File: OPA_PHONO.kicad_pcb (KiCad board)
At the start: 4 copper layers, 100 x 15 mm, 62 parts, among them J1 PJRAS2X1S01X, J2 PJRAS2X1S01X, J3 UJC-HP-3-SMT-TR, U1 OPA1644AxD, U2 OPA1612AxD, U3 LTC3265xDHC

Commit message: change output resistor to 499R
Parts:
- R12, R15, R24, R3, R6, R8: value 68R -> 499R
- R14, R19, R2, R7: value 2.32k -> 16k
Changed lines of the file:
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@@
     (descr "Resistor SMD 0402 (1005 Metric), square (rectangular) end terminal, IPC_7351 nominal, (Body size source: IPC-SM-782 page 72, https://www.pcb-3d.com/wordpress/wp-content/uploads/ipc-sm-782a_amendment_1_and_2.pdf), generated with kicad-footprint-generator")
     (tags "resistor")
-    (property "Description" "RES SMD 68 OHM 1% 1/16W 0402")
-    (property "MPN" "RT0402FRE0768RL")
+    (property "Description" "RES SMD 499R OHM 1% 1/16W 0402")
+    (property "MPN" "RT0402FRE07499RL")
     (property "Manufacturer" "YAGEO")
     (property "Sheetfile" "RIAA_PHONO.kicad_sch")
@@
       (effects (font (size 1 1) (thickness 0.15)))
     )
-    (fp_text value "68R" (at 0 1.17) (layer "F.Fab")
+    (fp_text value "499R" (at 0 1.17) (layer "F.Fab")
       (effects (font (size 1 1) (thickness 0.15)))
     )
@@
     (descr "Resistor SMD 0402 (1005 Metric), square (rectangular) end terminal, IPC_7351 nominal, (Body size source: IPC-SM-782 page 72, https://www.pcb-3d.com/wordpress/wp-content/uploads/ipc-sm-782a_amendment_1_and_2.pdf), generated with kicad-footprint-generator")
     (tags "resistor")
-    (property "Description" "RES SMD 2.32K OHM 1% 1/16W 0402")
-    (property "MPN" "RT0402FRE072K32L")
+    (property "Description" "RES SMD 16K OHM 1% 1/16W 0402")
+    (property "MPN" "RT0402FRE0716KL")
     (property "Manufacturer" "YAGEO")
     (property "Sheetfile" "RIAA_PHONO.kicad_sch")
@@
       (effects (font (size 1 1) (thickness 0.15)))
     )
-    (fp_text value "2.32k" (at 0 1.17 90) (layer "F.Fab")
+    (fp_text value "16k" (at 0 1.17 90) (layer "F.Fab")
       (effects (font (size 1 1) (thickness 0.15)))
     )
@@
     (descr "Resistor SMD 0402 (1005 Metric), square (rectangular) end terminal, IPC_7351 nominal, (Body size source: IPC-SM-782 page 72, https://www.pcb-3d.com/wordpress/wp-content/uploads/ipc-sm-782a_amendment_1_and_2.pdf), generated with kicad-footprint-generator")
     (tags "resistor")
-    (property "Description" "RES SMD 68 OHM 1% 1/16W 0402")
-    (property "MPN" "RT0402FRE0768RL")
+    (property "Description" "RES SMD 499R OHM 1% 1/16W 0402")
+    (property "MPN" "RT0402FRE07499RL")
     (property "Manufacturer" "YAGEO")
     (property "Sheetfile" "RIAA_PHONO.kicad_sch")
@@
       (effects (font (size 1 1) (thickness 0.15)))
     )
-    (fp_text value "68R" (at 0 1.17) (layer "F.Fab")
+    (fp_text value "499R" (at 0 1.17) (layer "F.Fab")
       (effects (font (size 1 1) (thickness 0.15)))
     )
@@
     (descr "Resistor SMD 0402 (1005 Metric), square (rectangular) end terminal, IPC_7351 nominal, (Body size source: IPC-SM-782 page 72, https://www.pcb-3d.com/wordpress/wp-content/uploads/ipc-sm-782a_amendment_1_and_2.pdf), generated with kicad-footprint-generator")
     (tags "resistor")
-    (property "Description" "RES SMD 2.32K OHM 1% 1/16W 0402")
-    (property "MPN" "RT0402FRE072K32L")
+    (property "Description" "RES SMD 16K OHM 1% 1/16W 0402")
+    (property "MPN" "RT0402FRE0716KL")
     (property "Manufacturer" "YAGEO")
     (property "Sheetfile" "RIAA_PHONO.kicad_sch")
@@
       (effects (font (size 1 1) (thickness 0.15)))
     )
-    (fp_text value "2.32k" (at 0 1.17) (layer "F.Fab")
+    (fp_text value "16k" (at 0 1.17) (layer "F.Fab")
       (effects (font (size 1 1) (thickness 0.15)))
     )
@@
     (descr "Resistor SMD 0402 (1005 Metric), square (rectangular) end terminal, IPC_7351 nominal, (Body size source: IPC-SM-782 page 72, https://www.pcb-3d.com/wordpress/wp-content/uploads/ipc-sm-782a_amendment_1_and_2.pdf), generated with kicad-footprint-generator")
     (tags "resistor")
-    (property "Description" "RES SMD 68 OHM 1% 1/16W 0402")
-    (property "MPN" "RT0402FRE0768RL")
+    (property "Description" "RES SMD 499R OHM 1% 1/16W 0402")
+    (property "MPN" "RT0402FRE07499RL")
     (property "Manufacturer" "YAGEO")
     (property "Sheetfile" "RIAA_PHONO.kicad_sch")
@@
       (effects (font (size 1 1) (thickness 0.15)))
     )
-    (fp_text value "68R" (at 0 1.17) (layer "F.Fab")
+    (fp_text value "499R" (at 0 1.17) (layer "F.Fab")
       (effects (font (size 1 1) (thickness 0.15)))
     )
@@
     (descr "Resistor SMD 0402 (1005 Metric), square (rectangular) end terminal, IPC_7351 nominal, (Body size source: IPC-SM-782 page 72, https://www.pcb-3d.com/wordpress/wp-content/uploads/ipc-sm-782a_amendment_1_and_2.pdf), generated with kicad-footprint-generator")
     (tags "resistor")
-    (property "Description" "RES SMD 68 OHM 1% 1/16W 0402")
-    (property "MPN" "RT0402FRE0768RL")
+    (property "Description" "RES SMD 499R OHM 1% 1/16W 0402")
+    (property "MPN" "RT0402FRE07499RL")
     (property "Manufacturer" "YAGEO")
     (property "Sheetfile" "RIAA_PHONO.kicad_sch")
@@
       (effects (font (size 1 1) (thickness 0.15)))
     )
-    (fp_text value "68R" (at 0 1.17 90) (layer "F.Fab")
+    (fp_text value "499R" (at 0 1.17 90) (layer "F.Fab")
       (effects (font (size 1 1) (thickness 0.15)))
     )
@@
     (descr "Resistor SMD 0402 (1005 Metric), square (rectangular) end terminal, IPC_7351 nominal, (Body size source: IPC-SM-782 page 72, https://www.pcb-3d.com/wordpress/wp-content/uploads/ipc-sm-782a_amendment_1_and_2.pdf), generated with kicad-footprint-generator")
     (tags "resistor")
-    (property "Description" "RES SMD 2.32K OHM 1% 1/16W 0402")
-    (property "MPN" "RT0402FRE072K32L")
+    (property "Description" "RES SMD 16K OHM 1% 1/16W 0402")
+    (property "MPN" "RT0402FRE0716KL")
     (property "Manufacturer" "YAGEO")
     (property "Sheetfile" "RIAA_PHONO.kicad_sch")
@@
       (effects (font (size 1 1) (thickness 0.15)))
     )
-    (fp_text value "2.32k" (at 0 1.17) (layer "F.Fab")
+    (fp_text value "16k" (at 0 1.17) (layer "F.Fab")
       (effects (font (size 1 1) (thickness 0.15)))
     )
@@
     (descr "Resistor SMD 0402 (1005 Metric), square (rectangular) end terminal, IPC_7351 nominal, (Body size source: IPC-SM-782 page 72, https://www.pcb-3d.com/wordpress/wp-content/uploads/ipc-sm-782a_amendment_1_and_2.pdf), generated with kicad-footprint-generator")
     (tags "resistor")
-    (property "Description" "RES SMD 68 OHM 1% 1/16W 0402")
-    (property "MPN" "RT0402FRE0768RL")
+    (property "Description" "RES SMD 499R OHM 1% 1/16W 0402")
+    (property "MPN" "RT0402FRE07499RL")
     (property "Manufacturer" "YAGEO")
     (property "Sheetfile" "RIAA_PHONO.kicad_sch")
@@
       (effects (font (size 1 1) (thickness 0.15)))
     )
-    (fp_text value "68R" (at 0 1.17) (layer "F.Fab")
+    (fp_text value "499R" (at 0 1.17) (layer "F.Fab")
       (effects (font (size 1 1) (thickness 0.15)))
     )
@@
     (descr "Resistor SMD 0402 (1005 Metric), square (rectangular) end terminal, IPC_7351 nominal, (Body size source: IPC-SM-782 page 72, https://www.pcb-3d.com/wordpress/wp-content/uploads/ipc-sm-782a_amendment_1_and_2.pdf), generated with kicad-footprint-generator")
     (tags "resistor")
-    (property "Description" "RES SMD 68 OHM 1% 1/16W 0402")
-    (property "MPN" "RT0402FRE0768RL")
+    (property "Description" "RES SMD 499R OHM 1% 1/16W 0402")
+    (property "MPN" "RT0402FRE07499RL")
     (property "Manufacturer" "YAGEO")
     (property "Sheetfile" "RIAA_PHONO.kicad_sch")
@@
       (effects (font (size 1 1) (thickness 0.15)))
     )
-    (fp_text value "68R" (at 0 1.17 90) (layer "F.Fab")
+    (fp_text value "499R" (at 0 1.17 90) (layer "F.Fab")
       (effects (font (size 1 1) (thickness 0.15)))
     )
@@
     (descr "Resistor SMD 0402 (1005 Metric), square (rectangular) end terminal, IPC_7351 nominal, (Body size source: IPC-SM-782 page 72, https://www.pcb-3d.com/wordpress/wp-content/uploads/ipc-sm-782a_amendment_1_and_2.pdf), generated with kicad-footprint-generator")
     (tags "resistor")
-    (property "Description" "RES SMD 2.32K OHM 1% 1/16W 0402")
-    (property "MPN" "RT0402FRE072K32L")
+    (property "Description" "RES SMD 16K OHM 1% 1/16W 0402")
+    (property "MPN" "RT0402FRE0716KL")
     (property "Manufacturer" "YAGEO")
     (property "Sheetfile" "RIAA_PHONO.kicad_sch")
@@
       (effects (font (size 1 1) (thickness 0.15)))
     )
-    (fp_text value "2.32k" (at 0 1.17 90) (layer "F.Fab")
-      (effects (font (size 1 1) (thickness 0.15)))
-    )
+    (fp_text value "16k" (at 0 1.17 90) (layer "F.Fab")
+      (effects (font (size 1 1) (thickness 0.15)))
+    )

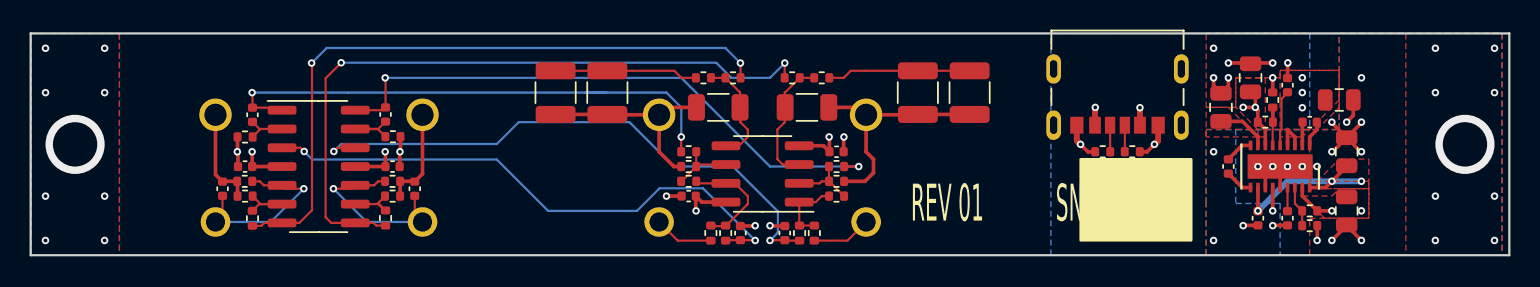
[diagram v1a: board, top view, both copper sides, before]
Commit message: Generate Gerbers
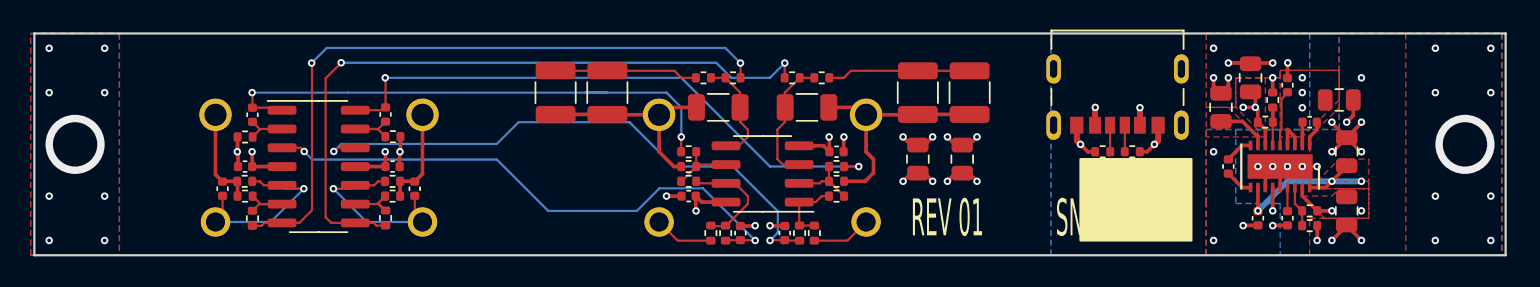
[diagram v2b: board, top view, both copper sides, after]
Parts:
- removed Ge: LOGO, LOGO
- added C15: 10u, Capacitor_SMD:C_0805_2012Metric, F.Cu at (160.0, 58.5)
- added C25: 10u, Capacitor_SMD:C_0805_2012Metric, F.Cu at (163.0, 58.5)
- added REF**: OSHW-Logo2_7.3x6mm_SilkScreen, Symbol:OSHW-Logo2_7.3x6mm_SilkScreen, B.Cu at (173.5, 54.0)
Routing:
- net GND: track 81.6 -> 86.5 mm, vias 51 -> 55
- net /POWER/+6V: track 9.23 -> 11.7 mm, vias 4 -> 6
- net /POWER/-6V: track 11.1 -> 13.6 mm, vias 4 -> 6
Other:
- board size 100 x 15 mm -> 99.5 x 15 mm
